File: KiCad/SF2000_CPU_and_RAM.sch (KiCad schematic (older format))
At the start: 1 part, among them U8 68000D

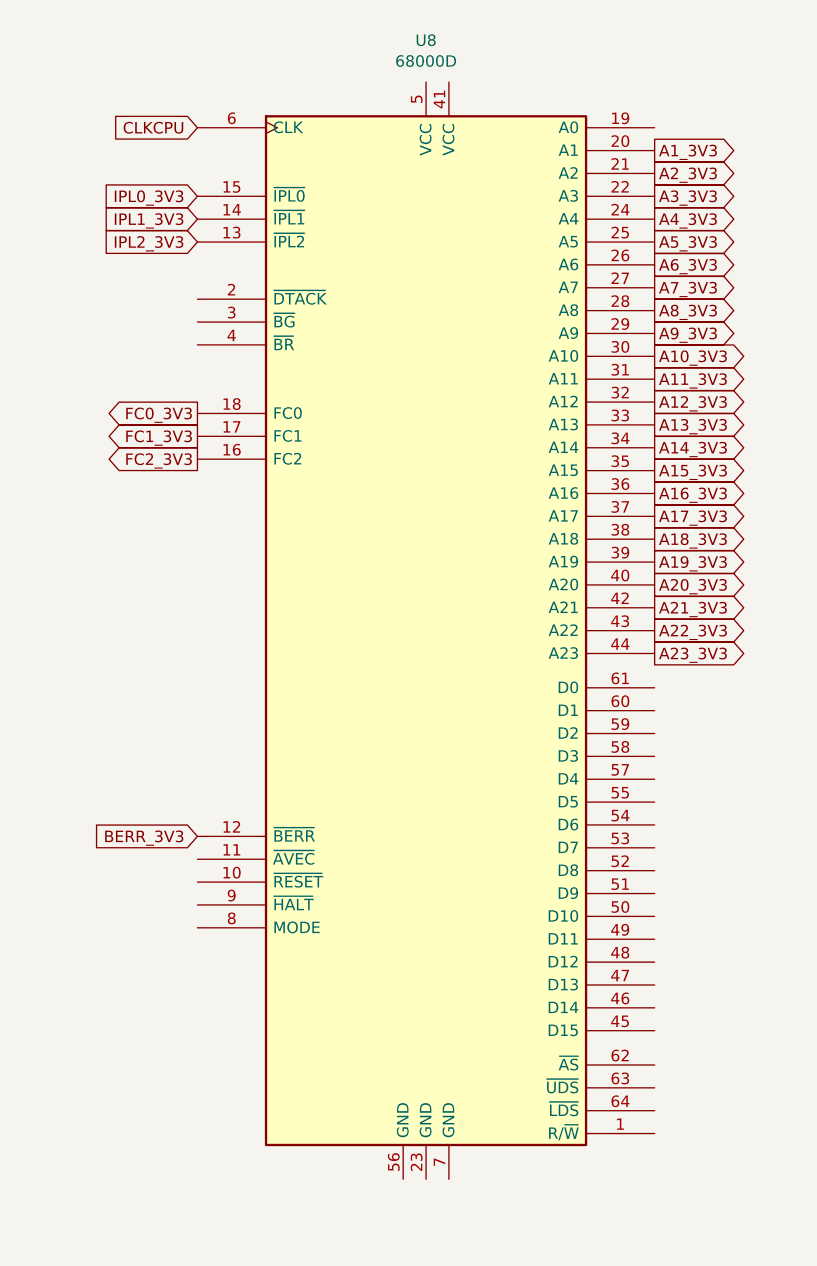
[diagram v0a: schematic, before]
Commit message: more dev, added nets
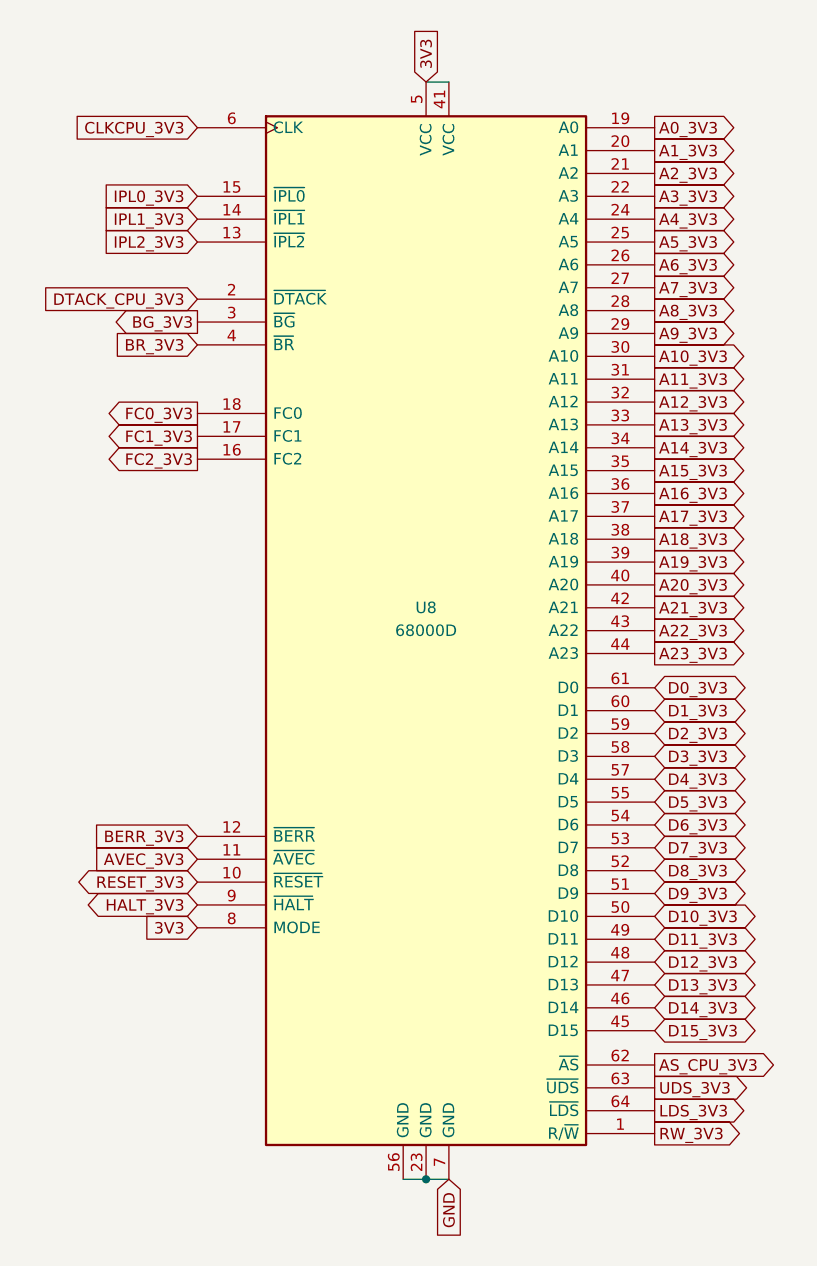
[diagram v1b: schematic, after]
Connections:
- net RW_3V3: now reaches U8.1 (R/~W)
- net RESET_3V3: now reaches U8.10 (~RESET)
- net AVEC_3V3: now reaches U8.11 (~AVEC)
- net A0_3V3: now reaches U8.19 (A0)
- net DTACK_CPU_3V3: now reaches U8.2 (~DTACK)
- net GND: now reaches U8.23 (GND)
- net GND: now also U8.56 (GND), U8.7 (GND)
- net BG_3V3: now reaches U8.3 (~BG)
- net BR_3V3: now reaches U8.4 (~BR)
- net 3V3: now reaches U8.41 (VCC)
- net 3V3: now also U8.5 (VCC), U8.8 (MODE)
- net D15_3V3: now reaches U8.45 (D15)
- net D14_3V3: now reaches U8.46 (D14)
- net D13_3V3: now reaches U8.47 (D13)
- net D12_3V3: now reaches U8.48 (D12)
- net D11_3V3: now reaches U8.49 (D11)
- net D10_3V3: now reaches U8.50 (D10)
- net D9_3V3: now reaches U8.51 (D9)
- net D8_3V3: now reaches U8.52 (D8)
- net D7_3V3: now reaches U8.53 (D7)
- net D6_3V3: now reaches U8.54 (D6)
- net D5_3V3: now reaches U8.55 (D5)
- net D4_3V3: now reaches U8.57 (D4)
- net D3_3V3: now reaches U8.58 (D3)
- net D2_3V3: now reaches U8.59 (D2)
- net D1_3V3: now reaches U8.60 (D1)
- net D0_3V3: now reaches U8.61 (D0)
- net AS_CPU_3V3: now reaches U8.62 (~AS)
- net UDS_3V3: now reaches U8.63 (~UDS)
- net LDS_3V3: now reaches U8.64 (~LDS)
- net HALT_3V3: now reaches U8.9 (~HALT)
- net CLKCPU renamed CLKCPU_3V3
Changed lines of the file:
@@
 U 1 1 621E09D7
 P 2500 3700
-F 0 "U8" H 2500 6281 50  0000 C CNN
-F 1 "68000D" H 2500 6190 50  0000 C CNN
+F 0 "U8" H 2500 3800 50  0000 C CNN
+F 1 "68000D" H 2500 3700 50  0000 C CNN
 F 2 "Package_QFP:LQFP-64_14x14mm_P0.8mm" H 2500 3700 50  0001 C CNN
 F 3 "https://www.nxp.com/docs/en/reference-manual/MC68000UM.pdf" H 2500 3700 50  0001 C CNN
@@
 $EndComp
 Text GLabel 1500 1500 0    50   Input ~ 0
-CLKCPU
+CLKCPU_3V3
 Text GLabel 3500 2000 2    50   Output ~ 0
 A5_3V3
@@
 Text GLabel 3500 3800 2    50   Output ~ 0
 A23_3V3
+Text GLabel 1500 2350 0    50   Output ~ 0
+BG_3V3
+Text GLabel 3500 1500 2    50   Output ~ 0
+A0_3V3
+Text GLabel 3500 3950 2    50   BiDi ~ 0
+D0_3V3
+Text GLabel 3500 4050 2    50   BiDi ~ 0
+D1_3V3
+Text GLabel 3500 4150 2    50   BiDi ~ 0
+D2_3V3
+Text GLabel 3500 4250 2    50   BiDi ~ 0
+D3_3V3
+Text GLabel 3500 4350 2    50   BiDi ~ 0
+D4_3V3
+Text GLabel 3500 4450 2    50   BiDi ~ 0
+D5_3V3
+Text GLabel 3500 4550 2    50   BiDi ~ 0
+D6_3V3
+Text GLabel 3500 4650 2    50   BiDi ~ 0
+D7_3V3
+Text GLabel 3500 4750 2    50   BiDi ~ 0
+D8_3V3
+Text GLabel 3500 4850 2    50   BiDi ~ 0
+D9_3V3
+Text GLabel 3500 4950 2    50   BiDi ~ 0
+D10_3V3
+Text GLabel 3500 5050 2    50   BiDi ~ 0
+D11_3V3
+Text GLabel 3500 5150 2    50   BiDi ~ 0
+D12_3V3
+Text GLabel 3500 5250 2    50   BiDi ~ 0
+D13_3V3
+Text GLabel 3500 5350 2    50   BiDi ~ 0
+D14_3V3
+Text GLabel 3500 5450 2    50   BiDi ~ 0
+D15_3V3
+Text GLabel 2500 1300 1    50   Input ~ 0
+3V3
+Wire Wire Line
+	2500 1300 2600 1300
+Text GLabel 1500 4700 0    50   Input ~ 0
+AVEC_3V3
+Text GLabel 1500 4800 0    50   BiDi ~ 0
+RESET_3V3
+Text GLabel 1500 4900 0    50   BiDi ~ 0
+HALT_3V3
+Text GLabel 1500 2450 0    50   Input ~ 0
+BR_3V3
+Text GLabel 1500 2250 0    50   Input ~ 0
+DTACK_CPU_3V3
+Text GLabel 2600 6100 3    50   Input ~ 0
+GND
+Wire Wire Line
+	2400 6100 2500 6100
+Connection ~ 2500 6100
+Wire Wire Line
+	2500 6100 2600 6100
+Text GLabel 3500 5600 2    50   Output ~ 0
+AS_CPU_3V3
+Text GLabel 3500 5700 2    50   Output ~ 0
+UDS_3V3
+Text GLabel 3500 5800 2    50   Output ~ 0
+LDS_3V3
+Text GLabel 3500 5900 2    50   Output ~ 0
+RW_3V3
+Text GLabel 1500 5000 0    50   Input ~ 0
+3V3
 $EndSCHEMATC
